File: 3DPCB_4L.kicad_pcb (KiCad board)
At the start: 4 copper layers, 100 x 60 mm, 758 parts, among them IC1 DRV8825, IC2 DRV8825, IC3 DRV8825, IC4 DRV8825, IC5 DRV8825, IC6 MP9943, J10 , J11 , J12 , J13 , J14 , J15 , J16 , J2 , J3 , J4 , J5 , J6 , J7 , J8 , J9 , K1 CONN_3, K2 CONN_3, K3 CONN_3, K4 CONN_3, K5 CONN_3, K6 CONN_3, K7 CONN_3, K8 CONN_3, K9 CONN_3, P1 CONN_8, P11 CONN_3X2, P12 CONN_3X2, P13 CONN_4, P2 CONN_8, P5 CONN_4, P6 CONN_4, P7 CONN_4, P8 CONN_2, P9 CONN_4, U1 CONN_4_LERCHE, U10 MICRO-SD, U11 IX4427, U12 MCP4728, U13 CONN_4_LERCHE, U15 SPST_MOMENTARY, U16 CONN_4_LERCHE, U17 IX4427, U2 SPST_MOMENTARY, U21 CONN_4_LERCHE, U22 CONN_4_LERCHE, U23 MCP4728, U24 IRFH7932, U25 CONN_4_LERCHE, U3 BSS84, U4 CONN_4_LERCHE, U5 IRFH7932, U6 LPC1768_TQFP100, U7 IRFH7932, U8 IRFH7932

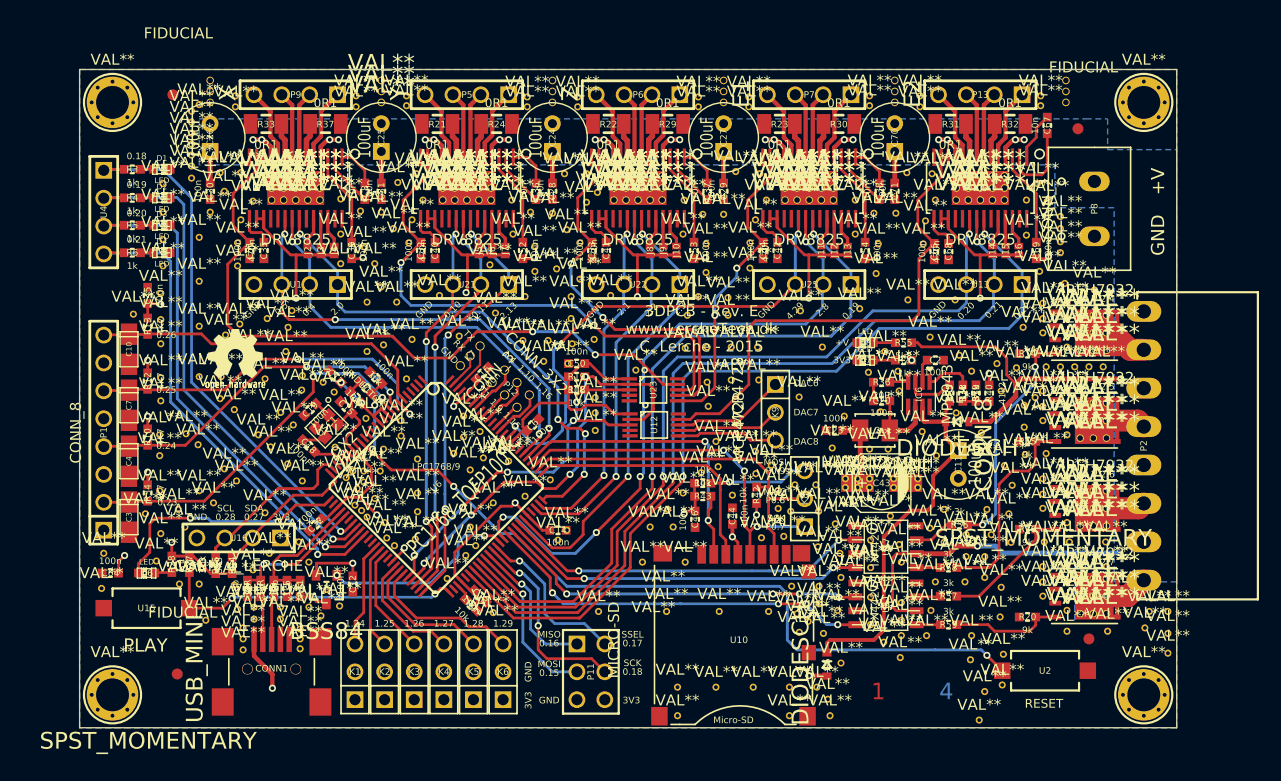
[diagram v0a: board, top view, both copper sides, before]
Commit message: Added LercheTech library
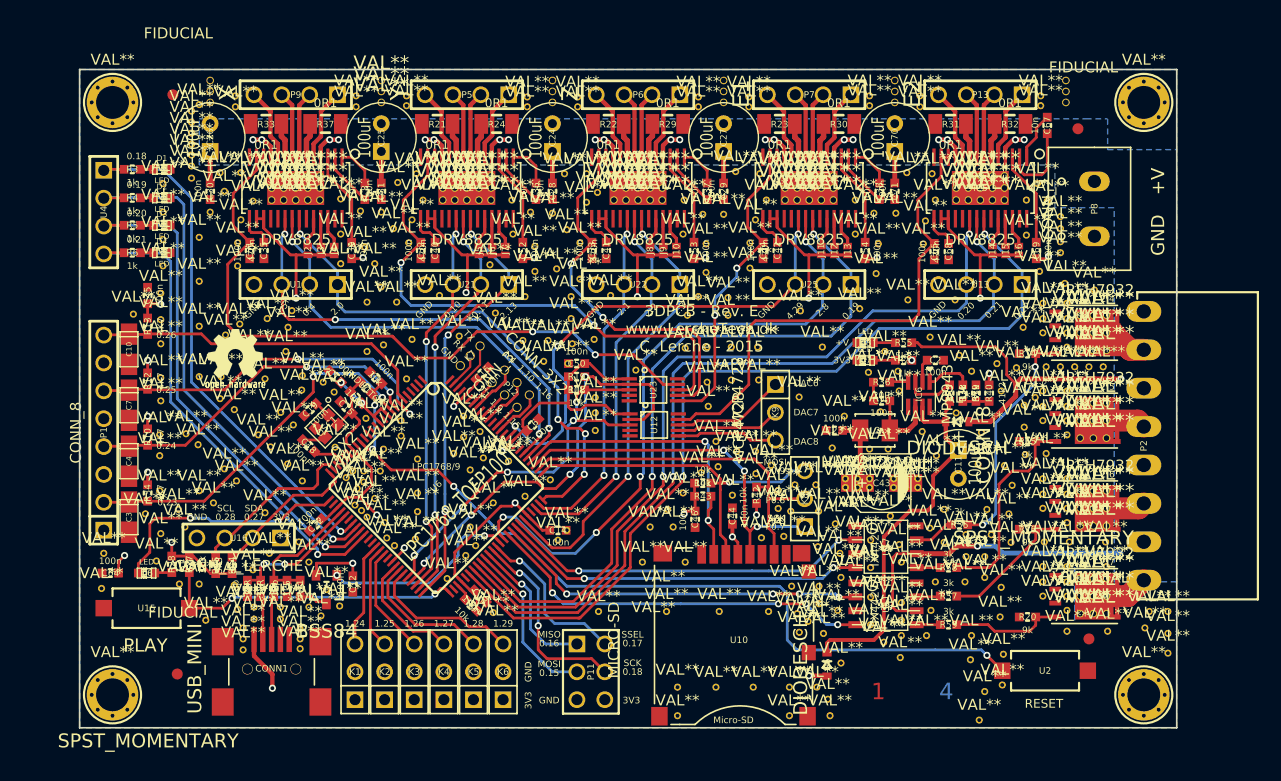
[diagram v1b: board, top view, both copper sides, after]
